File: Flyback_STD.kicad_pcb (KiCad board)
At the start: 2 copper layers, 23.8 x 22 mm, 28 parts, among them P1 VIN, P2 GND, P3 VOUT, P4 PGND, Q1 HSBA20N15S, U2 VPC2188B

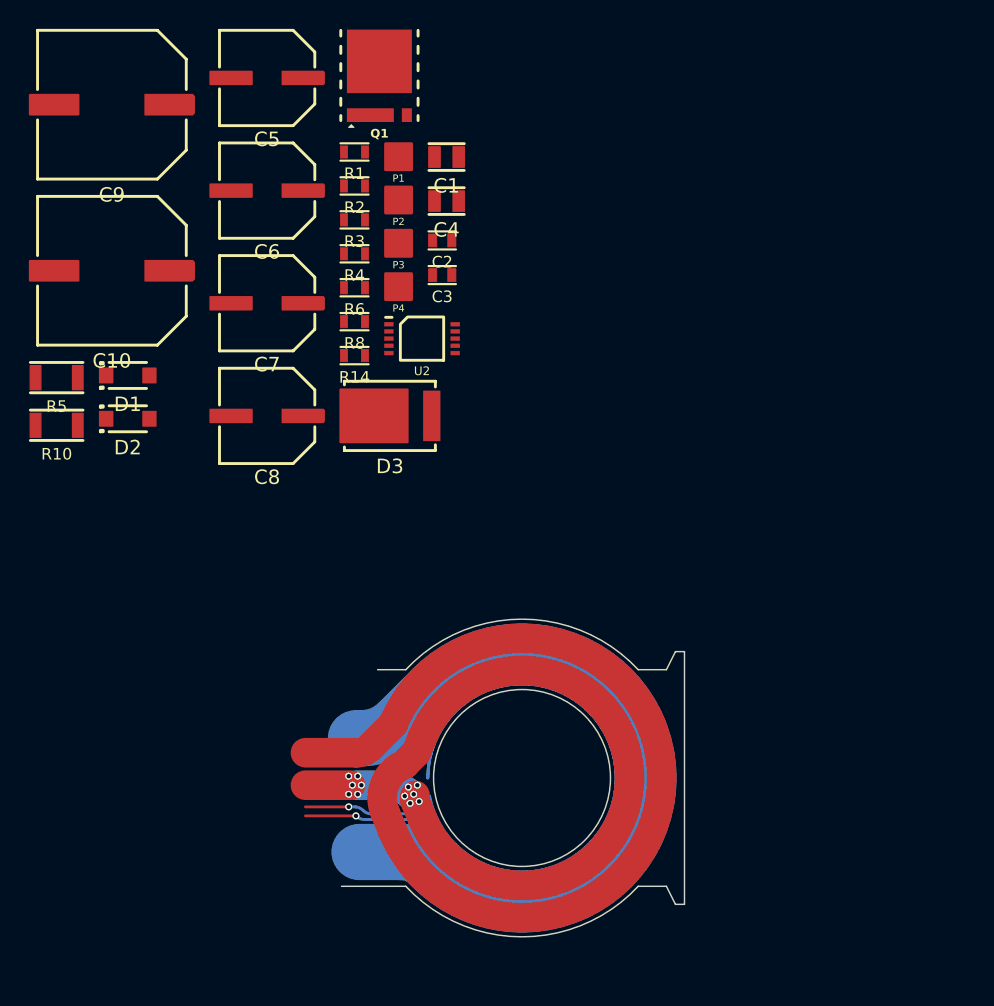
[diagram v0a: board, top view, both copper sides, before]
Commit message: Daily update
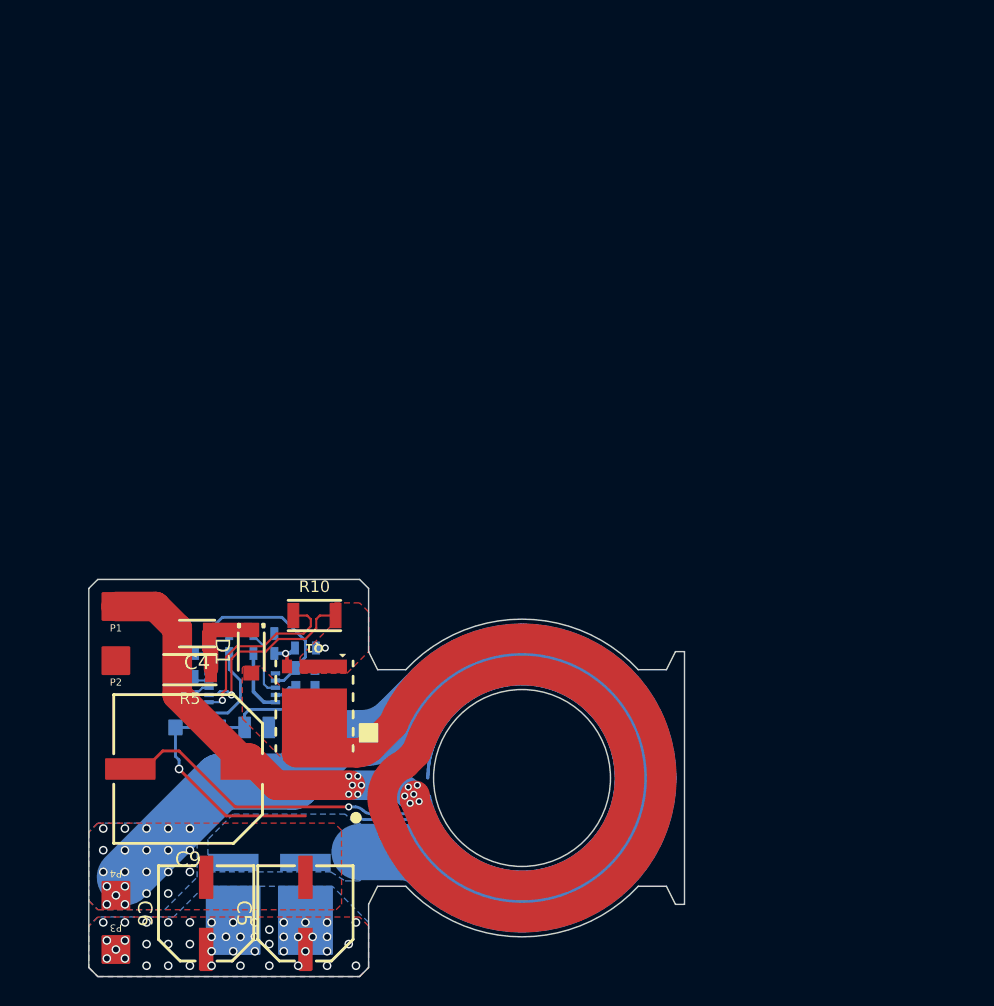
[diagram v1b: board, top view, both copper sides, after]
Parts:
- removed C10: 100uF, 007_GN_POLAR-CAP_SMD:CL-1010
- removed C8: 100uF, 007_GN_POLAR-CAP_SMD:CL-0608
- added D4: SB2080L, 102_SP_POWER_DIODE_SMD:TO-277A, B.Cu at (80.0, 108.8)
- C1, C3, D2, D3, R1, R14, R2, R3, R4, R6, R8, U2: moved to B.Cu
- C2: value 1uF -> 100nF; moved to B.Cu
- C7: value 100uF -> 100nF; footprint 007_GN_POLAR-CAP_SMD:CL-0608 -> 001_GN_RCL_SMD:C0603(1608M); moved to B.Cu
- moved C5 57.9 mm to (85.0, 109.4), turned to -90 degrees
- moved P3 52.7 mm to (71.9, 111.9), turned to 180 degrees
- moved C6 50.2 mm to (78.1, 109.4), turned to -90 degrees
- moved P4 46.5 mm to (71.9, 108.1), turned to 180 degrees
- moved C9 46.3 mm to (76.9, 99.4)
- moved Q1 43.9 mm to (85.6, 95.0), turned to 180 degrees
- moved C1 41.6 mm to (81.6, 96.5)
- moved P2 37.4 mm to (71.9, 91.9)
- moved P1 36.8 mm to (71.9, 88.1)
- moved R1 34.6 mm to (79.0, 90.0)
- moved C4 34.6 mm to (77.5, 90.0)
- moved D3 34.3 mm to (85.0, 108.8), turned to 90 degrees
- moved C3 33.1 mm to (76.6, 93.0), turned to 180 degrees
- moved R4 32.9 mm to (76.6, 94.4), turned to 180 degrees
- moved C2 32.4 mm to (85.0, 93.8)
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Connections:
- C7 pad 1: VDC -> VBUS
- C7 pad 2: GNDPWR -> GND
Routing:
- net GND: track 59.4 -> 104.7 mm, vias 2 -> 4
- net VBUS: track 115.2 -> 148.7 mm
- net GNDPWR: track 52.4 -> 72.4 mm, vias 0 -> 22
- net /CS: track 0.00 -> 13.7 mm, vias 0 -> 2
- net Vdrive: track 0.00 -> 9.24 mm
- net /UVP: track 0.00 -> 6.38 mm
- net Net-(D1-Cathode): track 0.00 -> 5.57 mm
- net /GT_U: track 0.00 -> 4.48 mm
- net /GT: track 0.00 -> 2.52 mm, vias 0 -> 1
- net Net-(U2-FB): track 0.00 -> 2.32 mm
- net /RT: track 0.00 -> 1.29 mm
- net /SS: track 0.00 -> 1.14 mm
- net VDC: vias 0 -> 46
- added copper zone on F.Cu, net /CS
- added copper zone on B.Cu, net GNDPWR
- added copper zone on F.Cu, net GNDPWR
- added copper zone on F.Cu, net VBUS
- added copper zone on B.Cu, net VDC
- added copper zone on F.Cu, net VDC
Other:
- board size 23.8 x 22 mm -> 41.2 x 27.5 mm

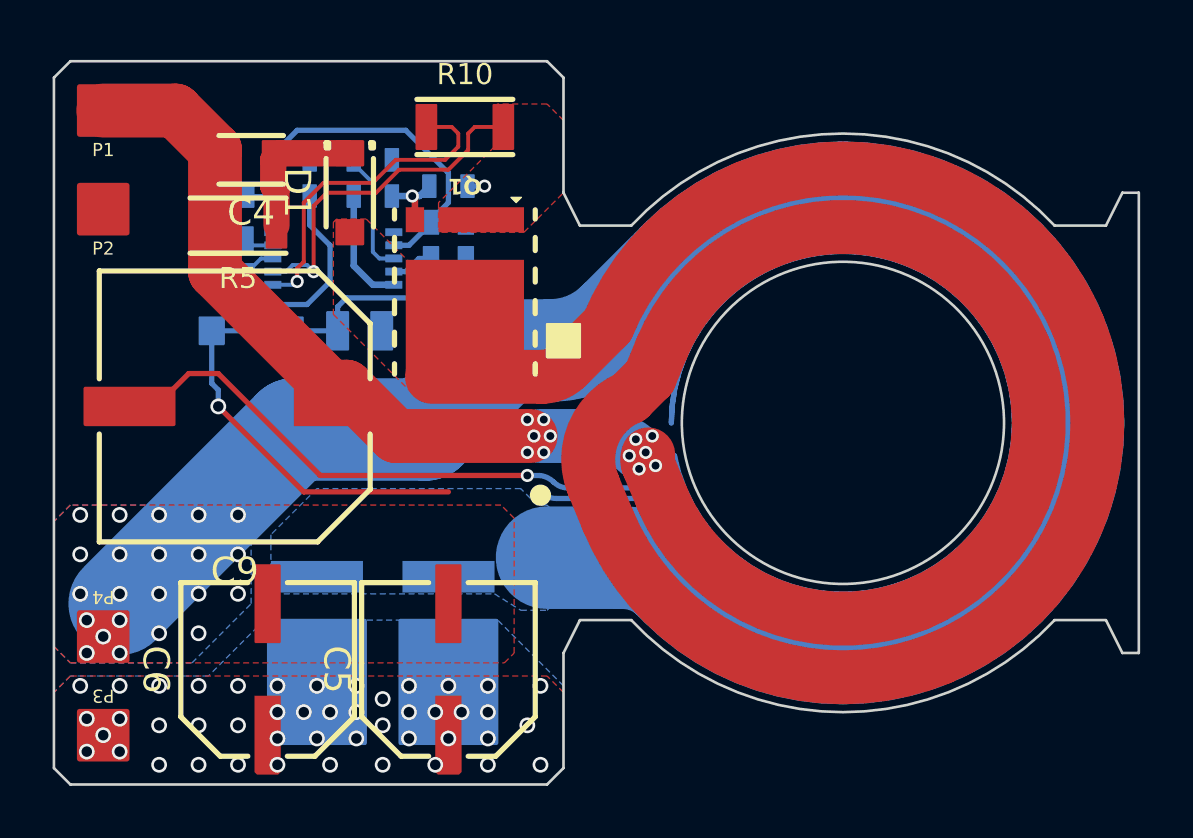
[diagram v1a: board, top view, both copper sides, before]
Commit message: Completed layout
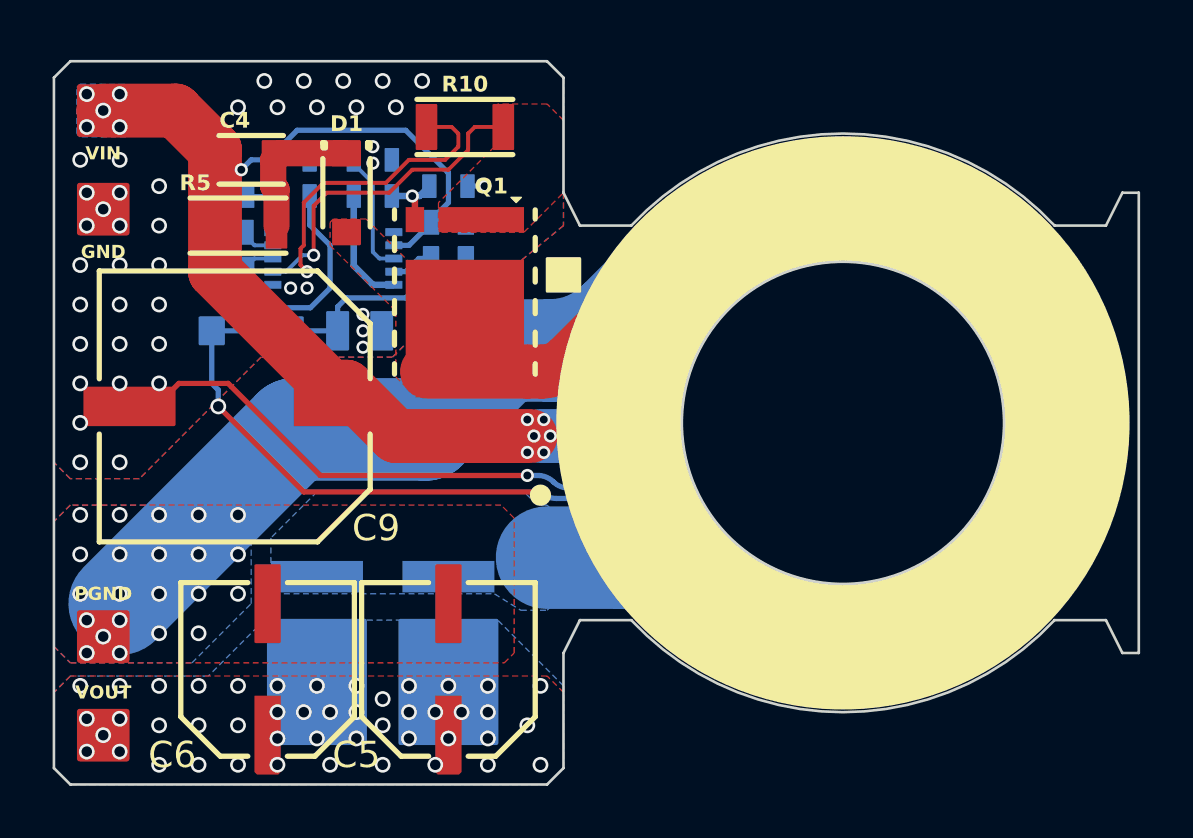
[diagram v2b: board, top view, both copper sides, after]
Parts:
- moved C3 0.25 mm to (76.6, 92.8)
- moved R4 0.25 mm to (76.6, 94.1)
- moved D1 0.12 mm to (81.1, 91.2)
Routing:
- net GND: track 104.7 -> 106.7 mm, vias 4 -> 45
- net VBUS: track 148.7 -> 150.7 mm, vias 12 -> 18
- net /CS: track 13.7 -> 13.2 mm
- added copper zone on B.Cu, net GND
- added copper zone on F.Cu, net GND
- added copper zone on B.Cu, net VBUS
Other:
- board text added: "Flyback_STD"
- board text added: "PkgLAN"
- board text added: "v0.9"

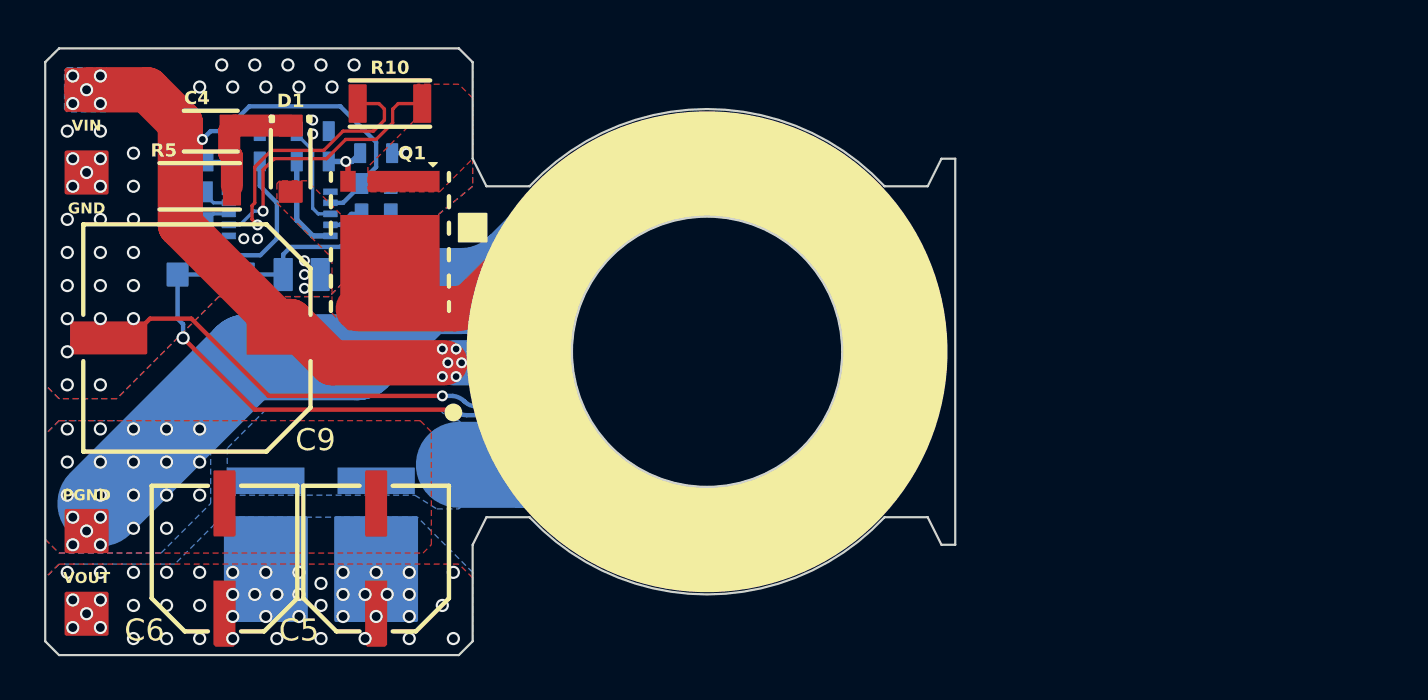
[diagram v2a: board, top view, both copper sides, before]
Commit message: Update to v0.9.1
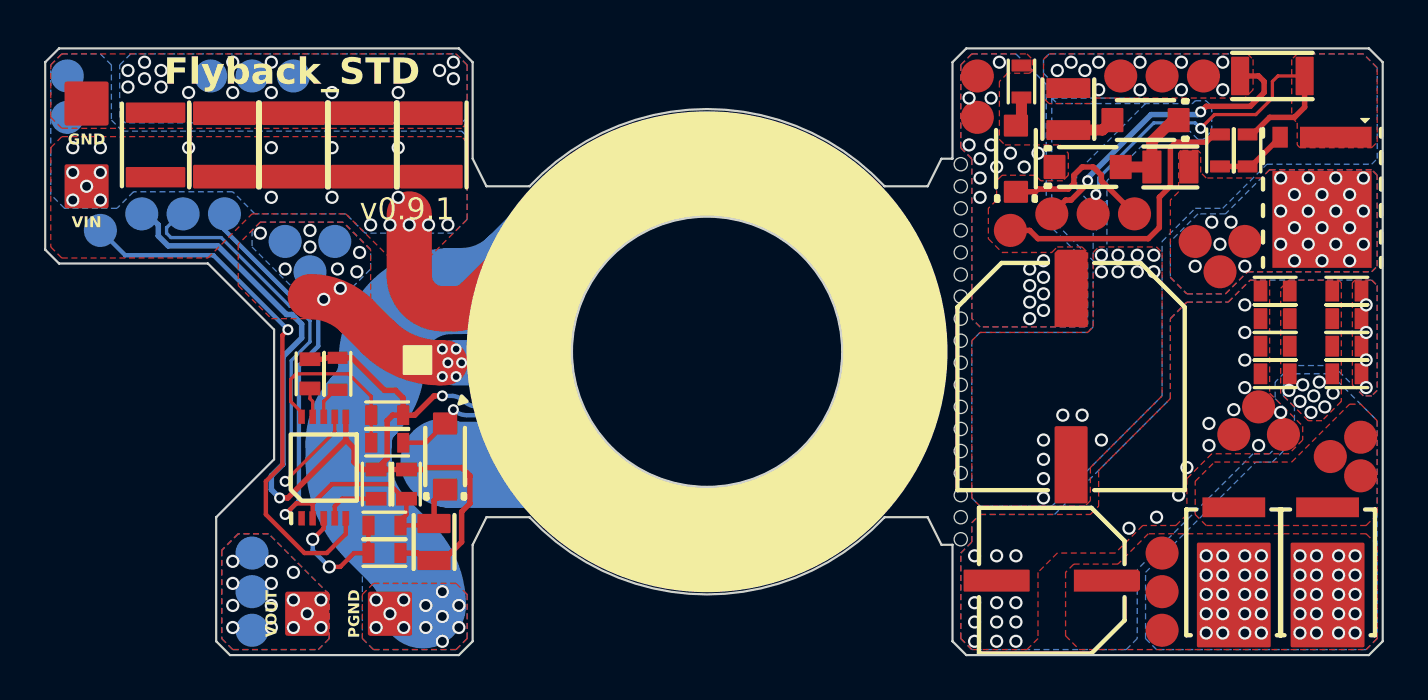
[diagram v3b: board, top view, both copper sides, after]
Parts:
- removed R14: 10k, 001_GN_RCL_SMD:R0603(1608M)
- removed U2: VPC2188B, 004_GN_MIDDLE-SEMI_SMD:MSOP-10_3030
- added C10: 10uF, 001_GN_RCL_SMD:C0805(2012M), F.Cu at (87.6, 108.6)
- added C11: 120uF, 007_GN_POLAR-CAP_SMD:CL-0608, F.Cu at (115.6, 110.4)
- added C12: 10uF, 001_GN_RCL_SMD:C0603(1608M), F.Cu at (125.8, 97.2)
- added C13: 10uF, 001_GN_RCL_SMD:C0603(1608M), F.Cu at (129.0, 97.2)
- added C14: 10uF, 001_GN_RCL_SMD:C0603(1608M), F.Cu at (125.8, 98.5)
- added C15: 10uF, 001_GN_RCL_SMD:C0603(1608M), F.Cu at (129.0, 98.5)
- added C16: 10uF, 001_GN_RCL_SMD:C0603(1608M), F.Cu at (125.8, 99.8)
- added C17: 10uF, 001_GN_RCL_SMD:C0603(1608M), F.Cu at (129.0, 99.8)
- added C18: 10uF, 001_GN_RCL_SMD:C0603(1608M), F.Cu at (125.8, 101.0)
- added C19: 10uF, 001_GN_RCL_SMD:C0603(1608M), F.Cu at (129.0, 101.0)
- added C8: 100uF, 007_GN_POLAR-CAP_SMD:CL-1010, F.Cu at (116.5, 101.1)
- added D5: SB2080L, 102_SP_POWER_DIODE_SMD:TO-277B, F.Cu at (128.1, 110.0)
- added D6: SB2080L, 102_SP_POWER_DIODE_SMD:TO-277B, F.Cu at (123.9, 110.0)
- added L1: 1uH, 008_GN_POWER-CHOKE_SMD:MC-2520, F.Cu at (116.4, 89.0)
- added R7: 10k, 001_GN_RCL_SMD:R0603(1608M), F.Cu at (124.5, 90.9)
- added R9: 36k, 001_GN_RCL_SMD:R0603(1608M), F.Cu at (85.5, 104.1)
- added REF**: NPTH-C_1006, 302_MECH_PAD:NPTH-C_1006, F.Cu at (111.5, 96.5)
- added REF**: NPTH-C_1006, 302_MECH_PAD:NPTH-C_1006, F.Cu at (111.5, 99.5)
- added REF**: SMP-C_15, 302_MECH_PAD:SMP-C_15, F.Cu at (128.2, 104.8)
- added REF**: NPTH-C_1006, 302_MECH_PAD:NPTH-C_1006, F.Cu at (111.5, 101.5)
- added REF**: NPTH-C_1006, 302_MECH_PAD:NPTH-C_1006, F.Cu at (111.5, 91.5)
- added REF**: SMP-C_15, 302_MECH_PAD:SMP-C_15, F.Cu at (120.6, 110.9)
- added REF**: NPTH-C_1006, 302_MECH_PAD:NPTH-C_1006, F.Cu at (111.5, 108.5)
- added REF**: SMP-C_15, 302_MECH_PAD:SMP-C_15, F.Cu at (129.6, 103.9)
- added REF**: SMP-C_15, 302_MECH_PAD:SMP-C_15, F.Cu at (123.2, 96.4)
- added REF**: SMP-C_15, 302_MECH_PAD:SMP-C_15, F.Cu at (119.4, 93.8)
- added REF**: SMP-C_15, 302_MECH_PAD:SMP-C_15, F.Cu at (124.4, 95.0)
- added REF**: SMP-C_15, 302_MECH_PAD:SMP-C_15, F.Cu at (123.9, 103.8)
- added REF**: SMP-C_15, 302_MECH_PAD:SMP-C_15, F.Cu at (125.0, 102.5)
- added REF**: SMP-C_15, 302_MECH_PAD:SMP-C_15, F.Cu at (112.2, 89.4)
- added REF**: SMP-C_15, 302_MECH_PAD:SMP-C_15, F.Cu at (113.8, 94.5)
- added REF**: NPTH-C_1006, 302_MECH_PAD:NPTH-C_1006, F.Cu at (111.5, 93.5)
- added REF**: NPTH-C_1006, 302_MECH_PAD:NPTH-C_1006, F.Cu at (111.5, 104.5)
- added REF**: SMP-C_15, 302_MECH_PAD:SMP-C_15, F.Cu at (120.6, 109.1)
- added REF**: SMP-C_15, 302_MECH_PAD:SMP-C_15, F.Cu at (112.2, 87.5)
- added REF**: SMP-C_15, 302_MECH_PAD:SMP-C_15, F.Cu at (120.6, 112.6)
- added REF**: SMP-C_15, 302_MECH_PAD:SMP-C_15, F.Cu at (122.1, 95.0)
- added REF**: NPTH-C_1006, 302_MECH_PAD:NPTH-C_1006, F.Cu at (111.5, 107.5)
- added REF**: NPTH-C_1006, 302_MECH_PAD:NPTH-C_1006, F.Cu at (111.5, 94.5)
- added REF**: SMP-C_15, 302_MECH_PAD:SMP-C_15, F.Cu at (117.5, 93.8)
- added REF**: NPTH-C_1006, 302_MECH_PAD:NPTH-C_1006, F.Cu at (111.5, 95.5)
- added REF**: NPTH-C_1006, 302_MECH_PAD:NPTH-C_1006, F.Cu at (111.5, 106.5)
- added REF**: NPTH-C_1006, 302_MECH_PAD:NPTH-C_1006, F.Cu at (111.5, 103.5)
- added REF**: NPTH-C_1006, 302_MECH_PAD:NPTH-C_1006, F.Cu at (111.5, 97.5)
- added REF**: SMP-C_15, 302_MECH_PAD:SMP-C_15, F.Cu at (126.1, 103.8)
- added REF**: NPTH-C_1006, 302_MECH_PAD:NPTH-C_1006, F.Cu at (111.5, 92.5)
- added REF**: SMP-C_15, 302_MECH_PAD:SMP-C_15, F.Cu at (115.6, 93.8)
- added REF**: NPTH-C_1006, 302_MECH_PAD:NPTH-C_1006, F.Cu at (111.5, 98.5)
- added REF**: SMP-C_15, 302_MECH_PAD:SMP-C_15, F.Cu at (122.5, 87.5)
- added REF**: NPTH-C_1006, 302_MECH_PAD:NPTH-C_1006, F.Cu at (111.5, 102.5)
- added REF**: SMP-C_15, 302_MECH_PAD:SMP-C_15, B.Cu at (77.5, 87.5)
- added REF**: SMP-C_15, 302_MECH_PAD:SMP-C_15, B.Cu at (79.4, 110.9)
- added REF**: SMP-C_15, 302_MECH_PAD:SMP-C_15, B.Cu at (82.0, 96.4)
- added REF**: SMP-C_15, 302_MECH_PAD:SMP-C_15, B.Cu at (74.4, 93.8)
- added REF**: SMP-C_15, 302_MECH_PAD:SMP-C_15, B.Cu at (71.0, 89.4)
- added REF**: SMP-C_15, 302_MECH_PAD:SMP-C_15, B.Cu at (79.4, 87.5)
- added REF**: SMP-C_15, 302_MECH_PAD:SMP-C_15, B.Cu at (79.4, 109.1)
- added REF**: SMP-C_15, 302_MECH_PAD:SMP-C_15, B.Cu at (80.9, 95.0)
- added REF**: SMP-C_15, 302_MECH_PAD:SMP-C_15, B.Cu at (84.9, 103.8)
- added REF**: SMP-C_15, 302_MECH_PAD:SMP-C_15, B.Cu at (76.2, 93.8)
- added REF**: SMP-C_15, 302_MECH_PAD:SMP-C_15, F.Cu at (120.6, 87.5)
- added REF**: SMP-C_15, 302_MECH_PAD:SMP-C_15, B.Cu at (78.1, 93.8)
- added REF**: SMP-C_15, 302_MECH_PAD:SMP-C_15, B.Cu at (81.2, 87.5)
- added REF**: SMP-C_15, 302_MECH_PAD:SMP-C_15, B.Cu at (87.0, 104.8)
- added REF**: SMP-C_15, 302_MECH_PAD:SMP-C_15, B.Cu at (79.4, 112.6)
- added REF**: SMP-C_15, 302_MECH_PAD:SMP-C_15, B.Cu at (83.8, 102.5)
- added REF**: SMP-C_15, 302_MECH_PAD:SMP-C_15, B.Cu at (72.5, 94.5)
- added REF**: SMP-C_15, 302_MECH_PAD:SMP-C_15, B.Cu at (71.0, 87.5)
- added REF**: SMP-C_15, 302_MECH_PAD:SMP-C_15, B.Cu at (83.1, 95.0)
- added REF**: SMP-C_15, 302_MECH_PAD:SMP-C_15, B.Cu at (88.4, 105.6)
- added REF**: SMP-C_15, 302_MECH_PAD:SMP-C_15, B.Cu at (82.6, 103.8)
- added REF**: SMP-C_15, 302_MECH_PAD:SMP-C_15, F.Cu at (129.6, 105.6)
- added REF**: SMP-C_15, 302_MECH_PAD:SMP-C_15, B.Cu at (88.4, 103.9)
- added REF**: SMP-C_15, 302_MECH_PAD:SMP-C_15, F.Cu at (118.8, 87.5)
- added REF**: NPTH-C_1006, 302_MECH_PAD:NPTH-C_1006, F.Cu at (111.5, 100.5)
- added REF**: NPTH-C_1006, 302_MECH_PAD:NPTH-C_1006, F.Cu at (111.5, 105.5)
- added U1: VPC2188B, 004_GN_MIDDLE-SEMI_SMD:MSOP-10_3030, F.Cu at (82.6, 105.2)
- C1: value 10uF -> 100nF; footprint 001_GN_RCL_SMD:C0805(2012M) -> 001_GN_RCL_SMD:C0603(1608M); moved to F.Cu
- C2, C3: moved to F.Cu
- C4: value 100pF -> 4.7uF; footprint 001_GN_RCL_SMD:C0805(2012M) -> 001_GN_RCL_SMD:C1210(3225M)
- C5, C6: value 100uF -> 4.7uF; footprint 007_GN_POLAR-CAP_SMD:CL-0608 -> 001_GN_RCL_SMD:C1210(3225M)
- C7: value 100nF -> 4.7uF; footprint 001_GN_RCL_SMD:C0603(1608M) -> 001_GN_RCL_SMD:C1210(3225M); moved to F.Cu
- C9: value 100uF -> 1nF; footprint 007_GN_POLAR-CAP_SMD:CL-1010 -> 001_GN_RCL_SMD:C0805(2012M)
- D2: value DS110W -> DS120W; moved to F.Cu
- D3: value SB2080L -> DS120W; footprint 102_SP_POWER_DIODE_SMD:TO-277A -> 002_GN_TWO-PIN_PLASTIC_SMD:SOD-123F; moved to F.Cu
- D4: value SB2080L -> DS110W; footprint 102_SP_POWER_DIODE_SMD:TO-277A -> 002_GN_TWO-PIN_PLASTIC_SMD:SOD-123F; moved to F.Cu
- Q1: value HSBA20N15S -> HY1420C2
- R1: value 100k -> 100R; moved to F.Cu
- R10: value 30mR/1W -> 3.9k; footprint 001_GN_RCL_SMD:R1206(3216M) -> 001_GN_RCL_SMD:R0603(1608M)
- R2: value 4.7k -> 100k; moved to F.Cu
- R3: value 39k -> 5.6k; moved to F.Cu
- R4: value 51k -> 27k; moved to F.Cu
- R5: value 3.3k -> RL1210A680K; footprint 001_GN_RCL_SMD:R1206(3216M) -> 001_GN_RCL_SMD:R1210(3225M)
- R6: value 3.9k -> 2.2R; moved to F.Cu
- R8: value 2.2R -> 25mR/1W; footprint 001_GN_RCL_SMD:R0603(1608M) -> 001_GN_RCL_SMD:R1206(3216M); moved to F.Cu
- moved R6 46.6 mm to (123.2, 90.9), turned to -90 degrees
- moved C9 44.8 mm to (121.0, 91.6)
- moved R8 43.7 mm to (125.6, 87.5), turned to 180 degrees
- moved Q1 42.3 mm to (127.9, 93.0)
- moved D2 40.0 mm to (117.2, 91.6), turned to 0 degrees
- moved D3 39.8 mm to (119.9, 89.5), turned to 180 degrees
- moved R1 35.3 mm to (114.2, 87.8), turned to 90 degrees
- moved D1 32.9 mm to (114.0, 91.2), turned to 90 degrees
- moved C6 19.8 mm to (84.4, 90.6), turned to 90 degrees
- moved C5 19.1 mm to (81.2, 90.6), turned to 90 degrees
- moved R3 18.9 mm to (85.4, 109.1), turned to 0 degrees
- moved R2 18.2 mm to (85.4, 107.9), turned to 180 degrees
- moved P4 14.3 mm to (85.6, 111.9), turned to -90 degrees
- moved R10 14.1 mm to (85.5, 102.9), turned to 0 degrees
- moved C2 12.3 mm to (86.4, 106.0), turned to 90 degrees
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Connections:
- C2 pad 1: Vdrive -> VDD
- C4 pad 2: Net-(D1-Cathode) -> GND
- C5 pad 1: VDC -> VBUS
- C5 pad 2: GNDPWR -> GND
- C6 pad 1: VDC -> VBUS
- C6 pad 2: GNDPWR -> GND
- C9 pad 1: VBUS -> Net-(D2-Anode)
- C9 pad 2: GND -> VBUS
- D1 pad 1: Net-(D1-Cathode) -> VDD
- D1 pad 2: VBUS -> Net-(D1-Anode)
- D2 pad 1: Vdrive -> VBUS
- D2 pad 2: GND -> Net-(D2-Anode)
- R1 pad 1: VBUS -> Net-(D1-Anode)
- R1 pad 2: /UVP -> VBUS
- R10 pad 1: /CS -> Net-(U1-FB)
- R2 pad 1: /UVP -> VDD
- R2 pad 2: GND -> /UVP
- R3 pad 1: GND -> /UVP
- R3 pad 2: Net-(U2-FB) -> GND
- R5 pad 1: VBUS -> GND
- R5 pad 2: Net-(D1-Cathode) -> VBUS
- R6 pad 1: Net-(U2-FB) -> /GT_U
- R6 pad 2: GND -> /GT
- R8 pad 1: /GT_U -> /CS
- R8 pad 2: /GT -> GND
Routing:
- net VDD: track 0.00 -> 34.9 mm, vias 0 -> 1
- net /GT_U: track 4.48 -> 38.0 mm, vias 0 -> 1
- net VBUS: track 150.7 -> 121.1 mm, vias 18 -> 86
- net /CS: track 13.2 -> 39.1 mm, vias 2 -> 3
- net GND: track 106.7 -> 117.3 mm, vias 45 -> 47
- net Net-(U1-FB): track 0.00 -> 8.19 mm
- net Vdrive: track 8.95 -> 2.56 mm
- net Net-(D1-Cathode): track 5.44 -> 0.00 mm
- net Net-(D2-Anode): track 0.00 -> 4.19 mm
- net Net-(U2-FB): track 2.32 -> 0.00 mm
- net Net-(D3-Anode): track 0.00 -> 2.19 mm
- net GNDPWR: track 72.4 -> 70.6 mm, vias 22 -> 41
- net Net-(D1-Anode): track 0.00 -> 1.38 mm
- net /GT: track 2.52 -> 3.27 mm, vias 1 -> 0
- net /UVP: track 6.38 -> 6.00 mm, vias 0 -> 2
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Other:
- board size 41.2 x 27.5 mm -> 60.6 x 27.5 mm
- board text added: "v0.9.1"
- board text removed: "v0.9"
